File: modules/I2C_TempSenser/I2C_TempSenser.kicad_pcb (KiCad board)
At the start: 2 copper layers, 100 x 100 mm, 10 parts, among them U1 TMP119AIYBGR, U2 PCA9306YZTR, U3 TPS7A2033DQN

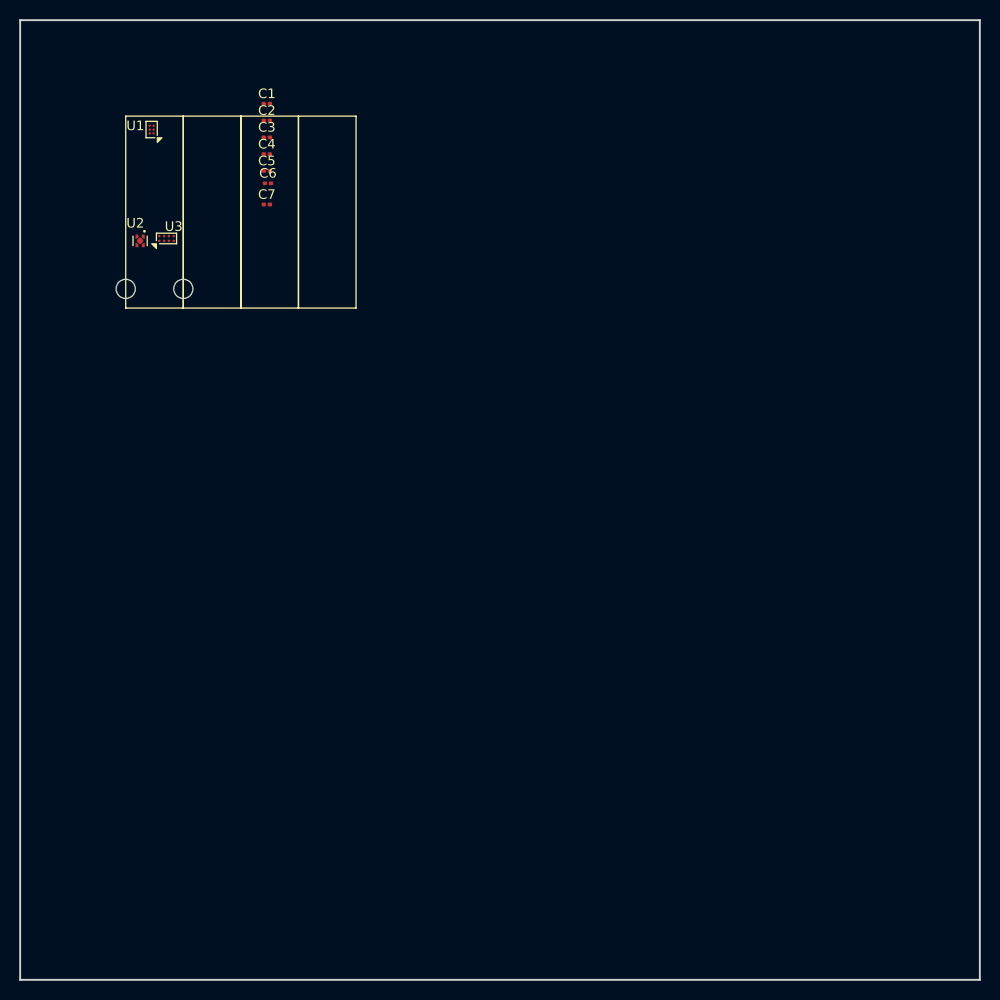
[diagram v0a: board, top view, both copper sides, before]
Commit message: update
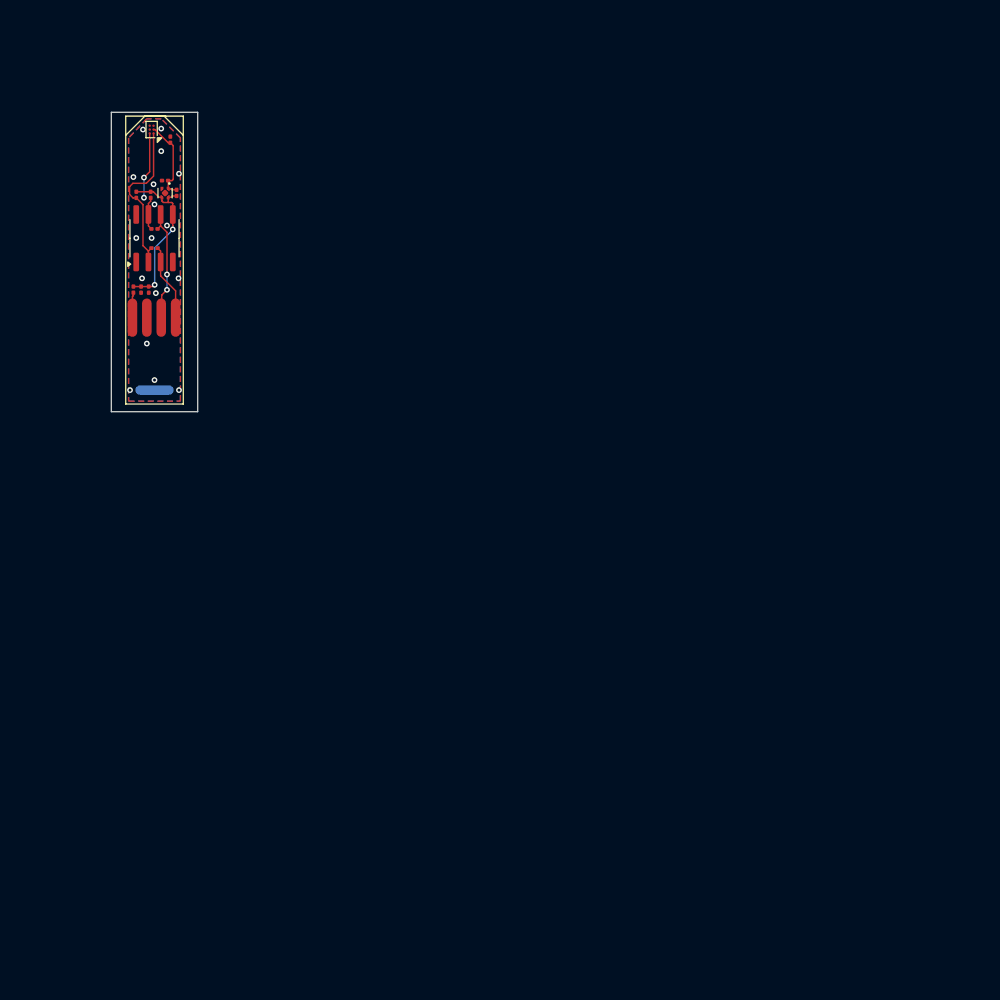
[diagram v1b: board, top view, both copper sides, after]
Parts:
- removed C1, C2, C3, C5, C7: 104C10, Capacitor_SMD:C_0201_0603Metric
- removed C6: 105C10, Capacitor_SMD:C_0201_0603Metric
- removed U2: PCA9306YZTR, Package_BGA:Texas_DSBGA-8_0.9x1.9mm_Layout2x4_P0.5mm
- added C101: 105C10, Capacitor_SMD:C_0201_0603Metric, F.Cu at (84.4, 68.1)
- added C102: 104C6P3, Capacitor_SMD:C_0201_0603Metric, F.Cu at (83.6, 68.1)
- added C104: 104C6P3, Capacitor_SMD:C_0201_0603Metric, F.Cu at (86.1, 56.7)
- added FB101: BLM03BX182SN1D, Inductor_SMD:L_0201_0603Metric, F.Cu at (82.8, 68.1)
- added R101: 0, Resistor_SMD:R_0201_0603Metric, F.Cu at (85.0, 63.8)
- added R102: 333C1S20, Resistor_SMD:R_0201_0603Metric, F.Cu at (83.1, 58.2)
- added R103: 0, Resistor_SMD:R_0201_0603Metric, F.Cu at (87.3, 58.0)
- added R104: 0, Resistor_SMD:R_0201_0603Metric, F.Cu at (85.0, 61.8)
- added R105: 333C1S20, Resistor_SMD:R_0201_0603Metric, F.Cu at (84.6, 58.2)
- added TP101: P5V, 0_Pad:Oval_Pad_1.0x4.0mm, F.Cu at (82.7, 71.0)
- added TP102: P5V, 0_Pad:Oval_Pad_1.0x4.0mm, F.Cu at (84.2, 71.0)
- added TP103: P5V, 0_Pad:Oval_Pad_1.0x4.0mm, F.Cu at (85.7, 71.0)
- added TP104: P5V, 0_Pad:Oval_Pad_1.0x4.0mm, F.Cu at (87.2, 71.0)
- added TP105: P5V, 0_Pad:Oval_Pad_1.0x4.0mm, B.Cu at (85.0, 78.5)
- added U102: P82B715DR, Package_SO:SOIC-8_3.9x4.9mm_P1.27mm, F.Cu at (85.0, 62.7)
- C103: renamed from C4; value 104C10 -> 104C6P3
- moved C103 10.2 mm to (86.7, 52.5), turned to 90 degrees
- moved U101 5.62 mm to (86.1, 58.0)
- renumbered U3 to U101, U1 to U103
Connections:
- U103 pad A1: /SCA2 -> /SDA1
- U103 pad A2: /SCL2 -> /SCL1
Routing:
- net +5V: track 0.00 -> 17.7 mm, vias 0 -> 2
- net /SDA1: track 0.00 -> 16.7 mm
- net /SCL2: track 0.00 -> 11.7 mm, vias 0 -> 2
- net /SCL1: track 0.00 -> 10.4 mm, vias 0 -> 2
- net +3.3V: track 0.00 -> 8.62 mm
- net /SDA2: track 0.00 -> 8.03 mm
- net Net-(FB101-Pad1): track 0.00 -> 2.54 mm
- net GND: vias 0 -> 17
- added copper zone on B.Cu, net GND
- added copper zone on F.Cu, net GND
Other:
- board size 100 x 100 mm -> 9 x 31.2 mm
